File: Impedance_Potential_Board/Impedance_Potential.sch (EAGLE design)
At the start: 39 parts, among them IC1 MAX30001GCWV+, U4 AP2112K-1.8V

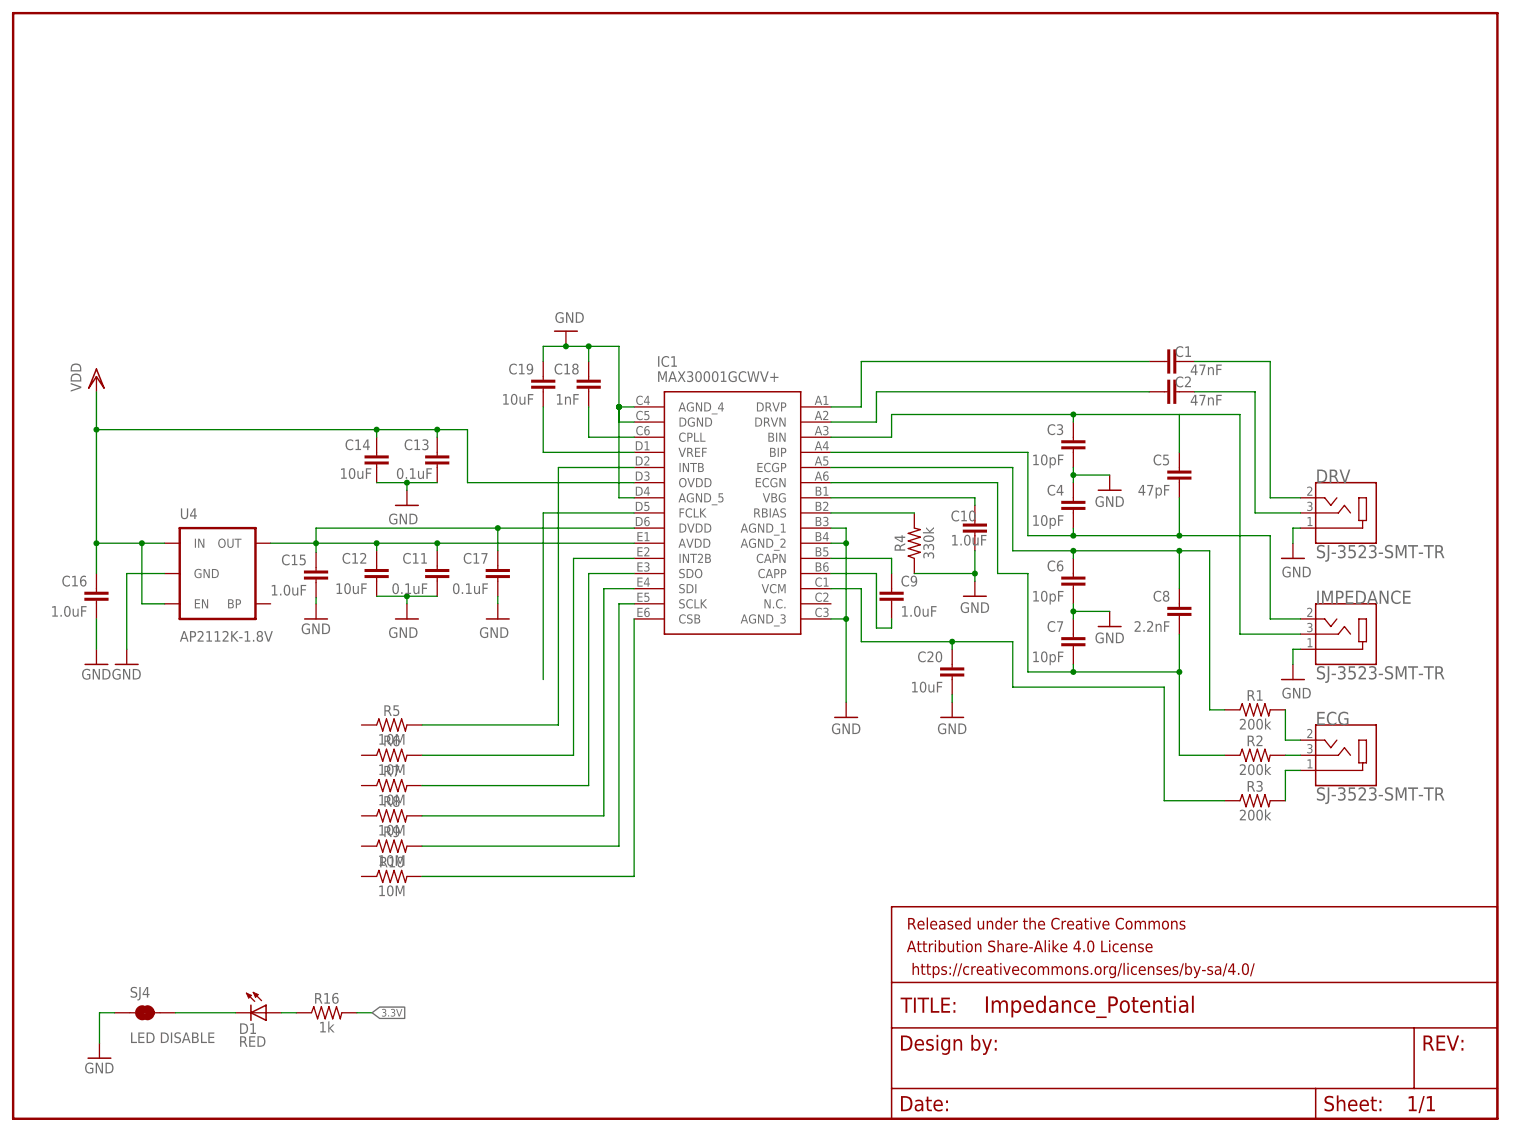
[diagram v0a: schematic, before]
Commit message: MAX30001G
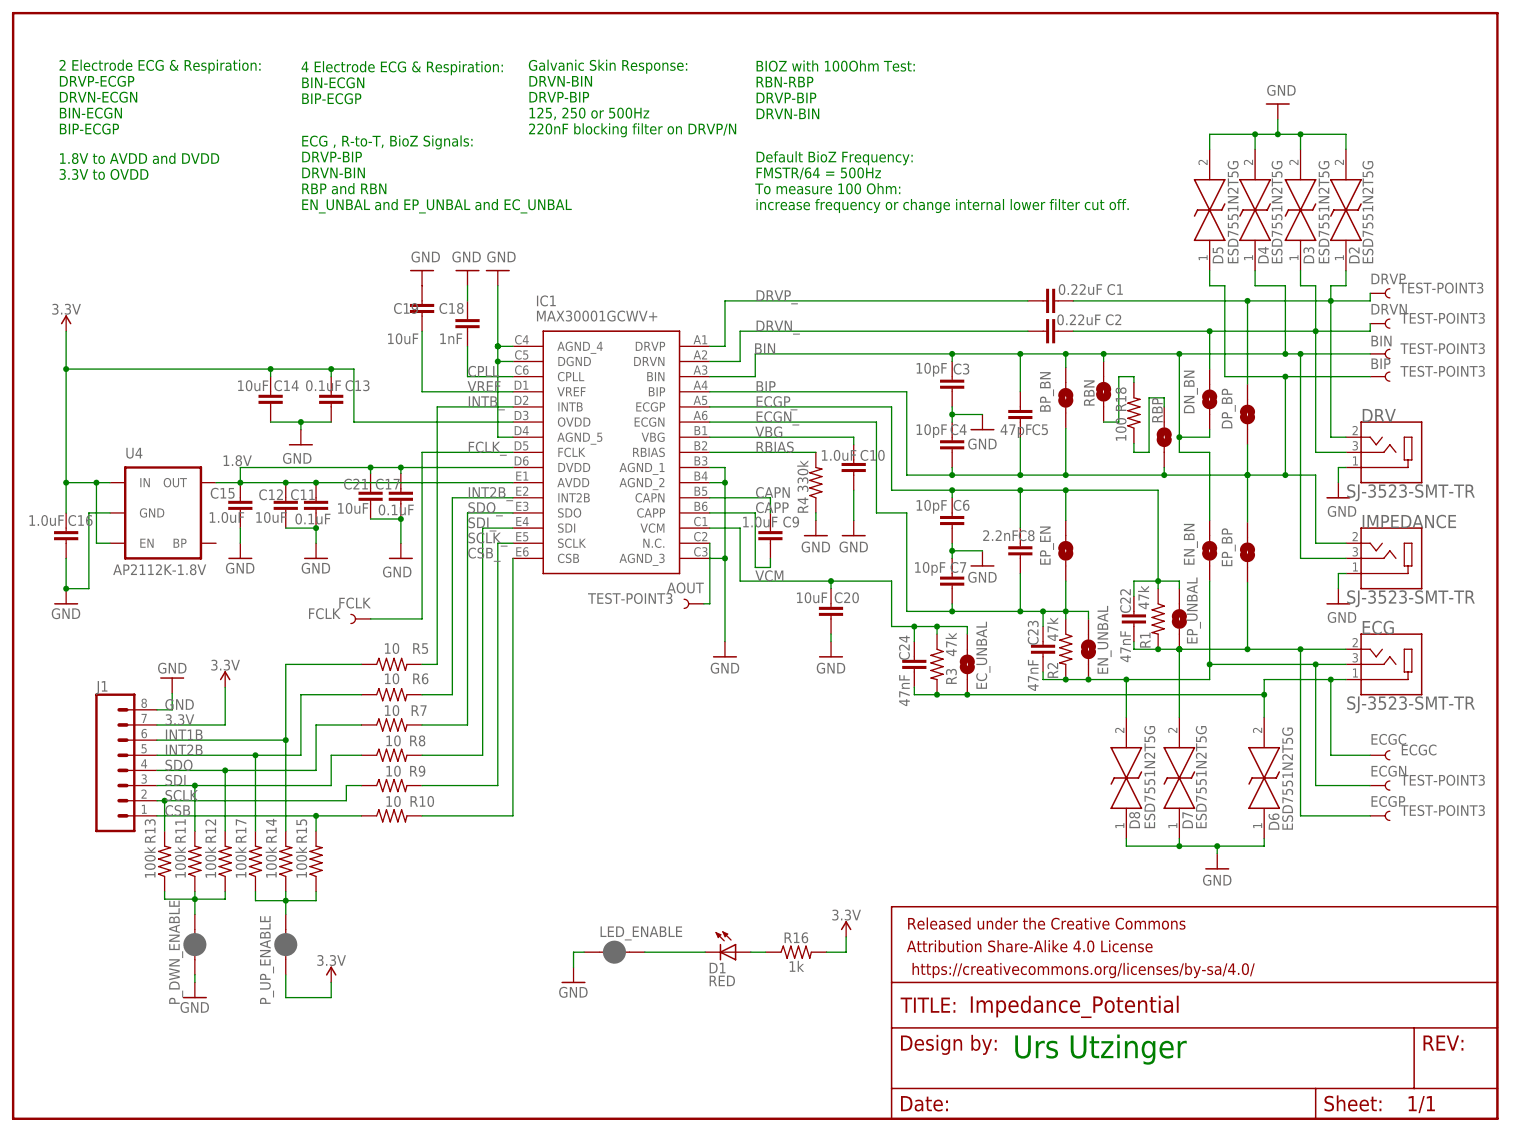
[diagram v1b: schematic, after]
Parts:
- removed SJ4: LED DISABLE, SparkFun-Jumpers:JUMPER-SMT_2_NC_TRACE_NO-SILK
- added AOUT, BIN, BIP, DRVN, DRVP, ECGN, ECGP: TEST-POINT3, SparkFun-Connectors:TEST-POINT3
- added BP_BN, DN_BN, DP_BP, EC_UNBAL, EN_BN, EN_UNBAL, EP_BP, EP_EN, EP_UNBAL, RBN, RBP: JUMPER-SMT_2_NO_SILK, SparkFun-Jumpers:JUMPER-SMT_2_NO_SILK
- added C21: 10uF, SparkFun-Capacitors:10UF-0603-6.3V-20%
- added C22, C23, C24: 47nF, SparkFun-Capacitors:47NF-0603-25V-5%
- added D2, D3, D4, D5, D6, D7, D8: ESD7551N2T5G, ESD7551N2T5G:ESD7551N2T5G
- added ECGC: ECGC, SparkFun-Connectors:TEST-POINT3
- added FCLK: FCLK, SparkFun-Connectors:TEST-POINT3
- added J1: (no value), SparkFun-Connectors:CONN_08"
- added LED_ENABLE: LED ENABLE, SparkFun-Jumpers:JUMPER-SMT_2_NC_PASTE_SILK
- added P_DWN_ENABLE, P_UP_ENABLE: JUMPER-SMT_2_NC_PASTE_SILK, SparkFun-Jumpers:JUMPER-SMT_2_NC_PASTE_SILK
- added R11, R12, R13, R14, R15, R17: 100k, SparkFun-Resistors:100KOHM-0603-1/10W-1%
- added R18: 100, SparkFun-Resistors:100OHM-0603-1/4W-5%
- C1, C2: value 47nF -> 0.22uF; device SparkFun-Capacitors:47NF-0603-25V-5% -> SparkFun-Capacitors:0.22UF-0603-25V-10%
- C11, C13, C17: device rcl:C-EUC0603 -> SparkFun-Capacitors:0.1UF-0603-25V-(+80/-20%)
- C12, C14, C19, C20: device rcl:C-EUC0603 -> SparkFun-Capacitors:10UF-0603-6.3V-20%
- R1, R2, R3: value 200k -> 47k; device SparkFun-Resistors:200KOHM-0603-1/10W-1% -> SparkFun-Resistors:47KOHM-0603-1/10W-1%
- R10, R5, R6, R7, R8, R9: value 10M -> 10; device SparkFun-Resistors:10MOHM-0603-1/10W-5% -> SparkFun-Resistors:10OHM-0603-1/10W-1%
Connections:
- net N$10 renamed CAPP
- net N$11 renamed CAPN
- net N$12 renamed VREF
- net N$16 renamed VBG
- net N$17 renamed RBIAS
- net N$18 renamed CSB_
- net N$2 renamed DRVP_
- net N$20 renamed CPLL
- net N$21 renamed SCLK_
- net N$22 renamed SDI_
- net N$23 renamed SDO_
- net N$24 renamed INT2B_
- net N$25 renamed INTB_
- net N$4 renamed DRVN_
- removed net N$1: C1.2, DRV.2
- removed net N$13: C3.1, C5.1, IC1.BIN, IMPEDANCE.3
- removed net N$14: ECG.3, R2.2
- removed net N$15: C7.2, C8.2, IC1.ECGN, R2.1
- removed net N$19: C11.1, C12.1, C15.2, C17.1, IC1.AVDD, IC1.DVDD, U4.OUT
- removed net N$27: IC1.FCLK
- removed net N$3: ECG.2, R1.2
- removed net N$5: C2.2, DRV.3
- removed net N$6: C4.2, C5.2, IC1.BIP, IMPEDANCE.2
- removed net N$7: ECG.1, R3.2
- removed net N$8: C20.1, IC1.VCM, R3.1
- removed net N$9: C6.1, C8.1, IC1.ECGP, R1.1
- removed net VDD: C13.1, C14.1, C16.2, IC1.OVDD, U4.EN, U4.IN
- new net 1.8V: C11.1, C12.1, C15.2, C17.1, C21.1, IC1.AVDD, IC1.DVDD, U4.OUT
- new net AOUT: AOUT.1, IC1.N.C.
- new net BIN: BIN.1, BP_BN.2, C3.1, C5.1, D4.1, DN_BN.1, EN_BN.2, IC1.BIN, IMPEDANCE.3, RBN.2
- new net BIP: BIP.1, BP_BN.1, C4.2, C5.2, D5.1, DP_BP.1, EP_BP.2, IC1.BIP, IMPEDANCE.2, RBP.1
- new net CSB: J1.1, R10.1, R15.2
- new net DRVN: C2.2, D3.1, DN_BN.2, DRV.3, DRVN.1
- new net DRVP: C1.2, D2.1, DP_BP.2, DRV.2, DRVP.1
- new net ECGC: C24.2, D6.2, ECG.1, ECGC.1, EC_UNBAL.1, R3.2
- new net ECGN: C23.2, D8.2, ECG.3, ECGN.1, EN_BN.1, EN_UNBAL.1, R2.2
- new net ECGN_: C23.1, C7.2, C8.2, EN_UNBAL.2, EP_EN.1, IC1.ECGN, R2.1
- new net ECGP: C22.2, D7.2, ECG.2, ECGP.1, EP_BP.1, EP_UNBAL.1, R1.2
- new net ECGP_: C22.1, C6.1, C8.1, EP_EN.2, EP_UNBAL.2, IC1.ECGP, R1.1
- new net FCLK_: FCLK.1, IC1.FCLK
- new net INT1B: J1.6, R14.2, R5.1
- new net INT2B: J1.5, R17.2, R6.1
- new net N$29: P_DWN_ENABLE.2, R11.1, R12.1, R13.1
- new net N$30: P_UP_ENABLE.2, R14.1, R15.1, R17.1
- new net N$32: R18.2, RBN.1
- new net N$33: R18.1, RBP.2
- new net SCLK: J1.2, R13.2, R9.1
- new net SDI: J1.3, R11.2, R8.1
- new net SDO: J1.4, R12.2, R7.1
- new net VCM: C20.1, C24.1, EC_UNBAL.2, IC1.VCM, R3.1
- net 3.3V: now also C13.1, C14.1, C16.2, IC1.OVDD, J1.7, P_UP_ENABLE.1, U4.EN, U4.IN
- net GND: now also C21.2, D2.2, D3.2, D4.2, D5.2, D6.1, D7.1, D8.1, J1.8, LED_ENABLE.1, P_DWN_ENABLE.1; no longer SJ4.1
- net N$28: now also LED_ENABLE.2; no longer SJ4.2
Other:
- note added: "1.8V to AVDD and DVDD 3.3V to OVDD"
- note added: "2 Electrode ECG & Respiration: DRVP-ECGP DRVN-ECGN BIN-ECGN BIP-ECGP"
- note added: "4 Electrode ECG & Respiration: BIN-ECGN BIP-ECGP"
- note added: "BIOZ with 100Ohm Test: RBN-RBP DRVP-BIP DRVN-BIN"
- note added: "Default BioZ Frequency: FMSTR/64 = 500Hz To measure 100 Ohm: increase frequency or change internal lower filter cut off."
- note added: "ECG , R-to-T, BioZ Signals: DRVP-BIP DRVN-BIN RBP and RBN EN_UNBAL and EP_UNBAL and EC_UNBAL"
- note added: "Galvanic Skin Response: DRVN-BIN DRVP-BIP 125, 250 or 500Hz 220nF blocking filter on DRVP/N"
- note added: "Urs Utzinger"
- moved on the sheet: C1, C10, C11, C12, C13, C14, C15, C16, C17, C18, C19, C2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
